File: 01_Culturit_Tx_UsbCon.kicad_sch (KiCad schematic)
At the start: 20 parts, among them CN1 2.54 X 2P, J2 USB4105-GF-A, U1 MAX1555EZK+T, U2 BQ27441DRZR-G1A

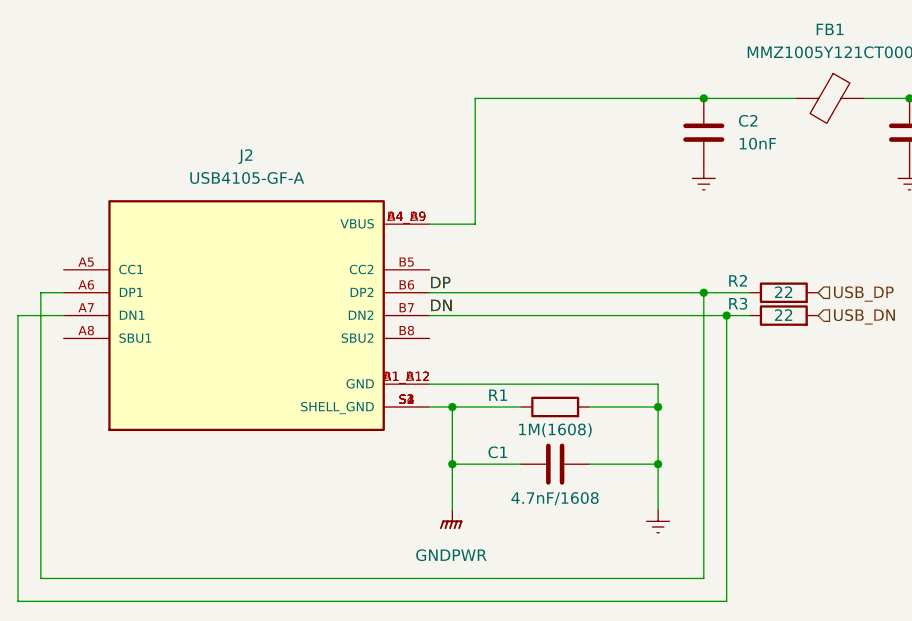
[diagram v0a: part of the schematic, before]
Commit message: 2022-11-01
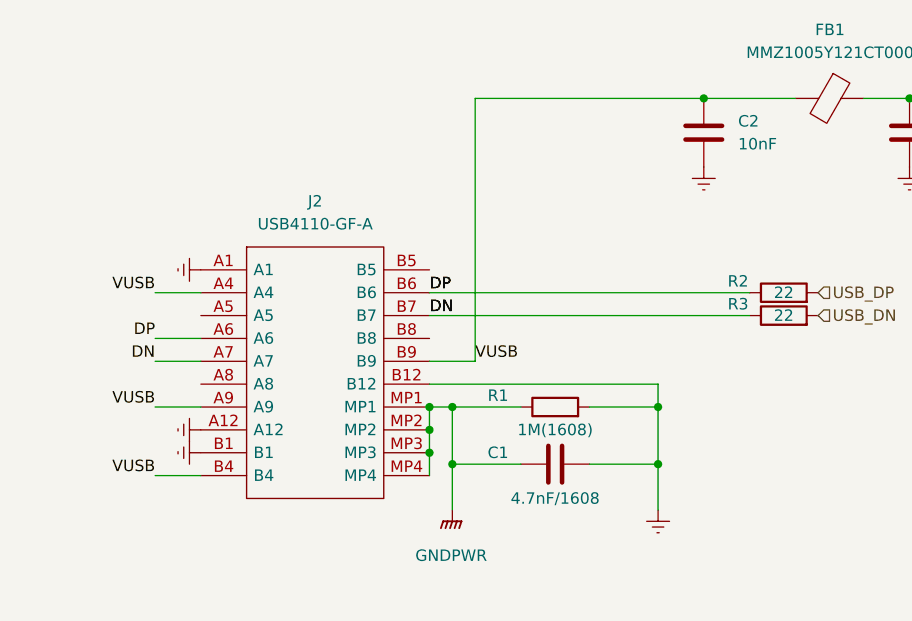
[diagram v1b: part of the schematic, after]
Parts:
- removed J2: USB4105-GF-A, Local_devices:GCT_USB4105-GF-A, symbol USB4105-GF-A:USB4105-GF-A
- added J2: USB4110-GF-A, Local_devices:USB4110GFA, symbol USB4110-GF-A:USB4110-GF-A
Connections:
- net DN: now also J2.A7, J2.B7
- net DP: now also J2.A6, J2.B6
- net Earth: now also J2.A1, J2.A12, J2.B1, J2.B12
- net GNDPWR: now also J2.MP1, J2.MP2, J2.MP3, J2.MP4
- net VUSB: now reaches C2.1, FB1.2
- net VUSB: now also J2.A4, J2.A9, J2.B4, J2.B9
